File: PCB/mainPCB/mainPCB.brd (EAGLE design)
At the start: 98.7 x 80 mm, 58 parts, among them CN1 SDS-50J, CN2 SDS-50J, CN3 SDS-50J, CN4 SDS-50J, J2 RASPBERRYPI-40-PIN-GPIO, T2 BC817, T3 BC817, T4 BC817, T6 BC817, U1 AT24C256C-SSHL-B, U11 SFH615A-07, U12 ALQ105, U3 SFH615A-07, U4 ALQ105, U5 SFH615A-07, U6 ALQ105, U7 SFH615A-07, U8 ALQ105

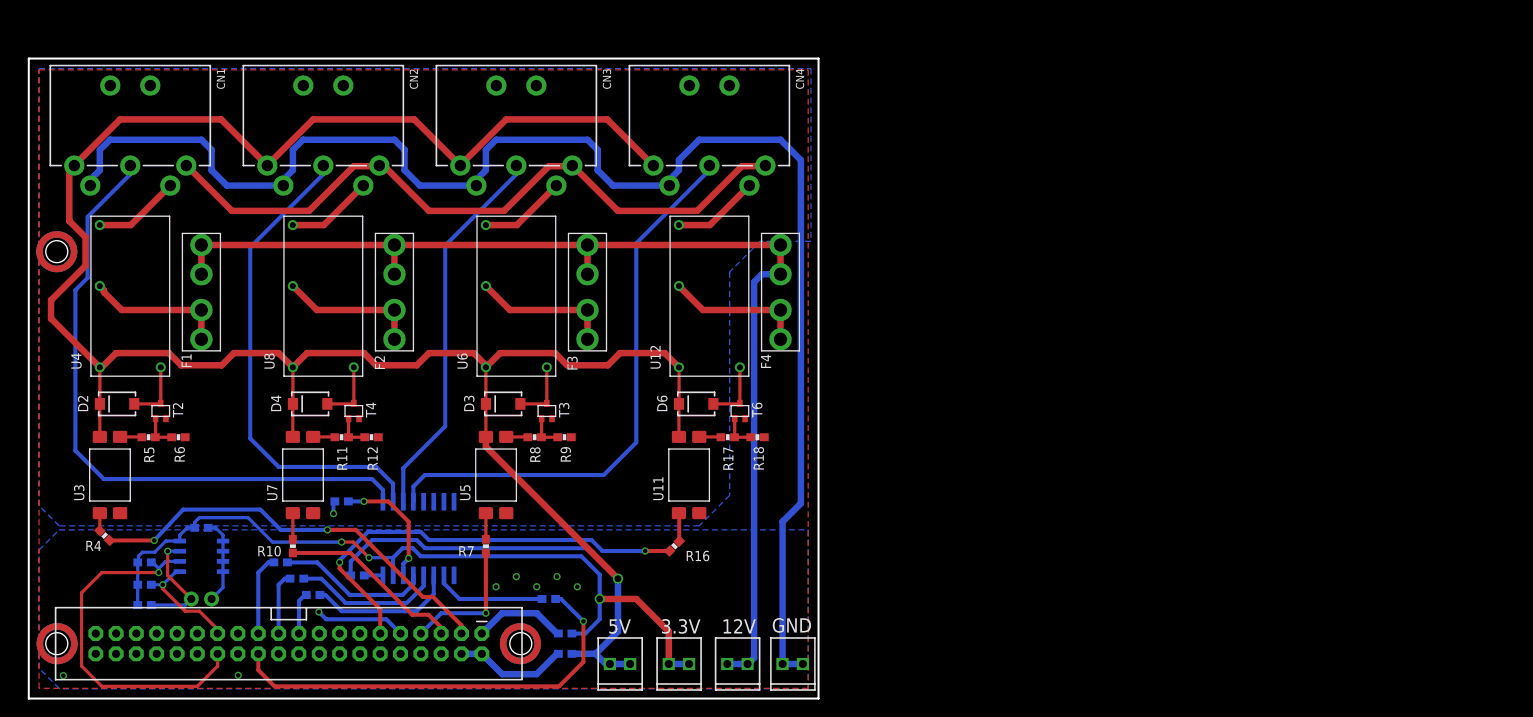
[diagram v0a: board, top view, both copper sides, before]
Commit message: Adding files for v0.2
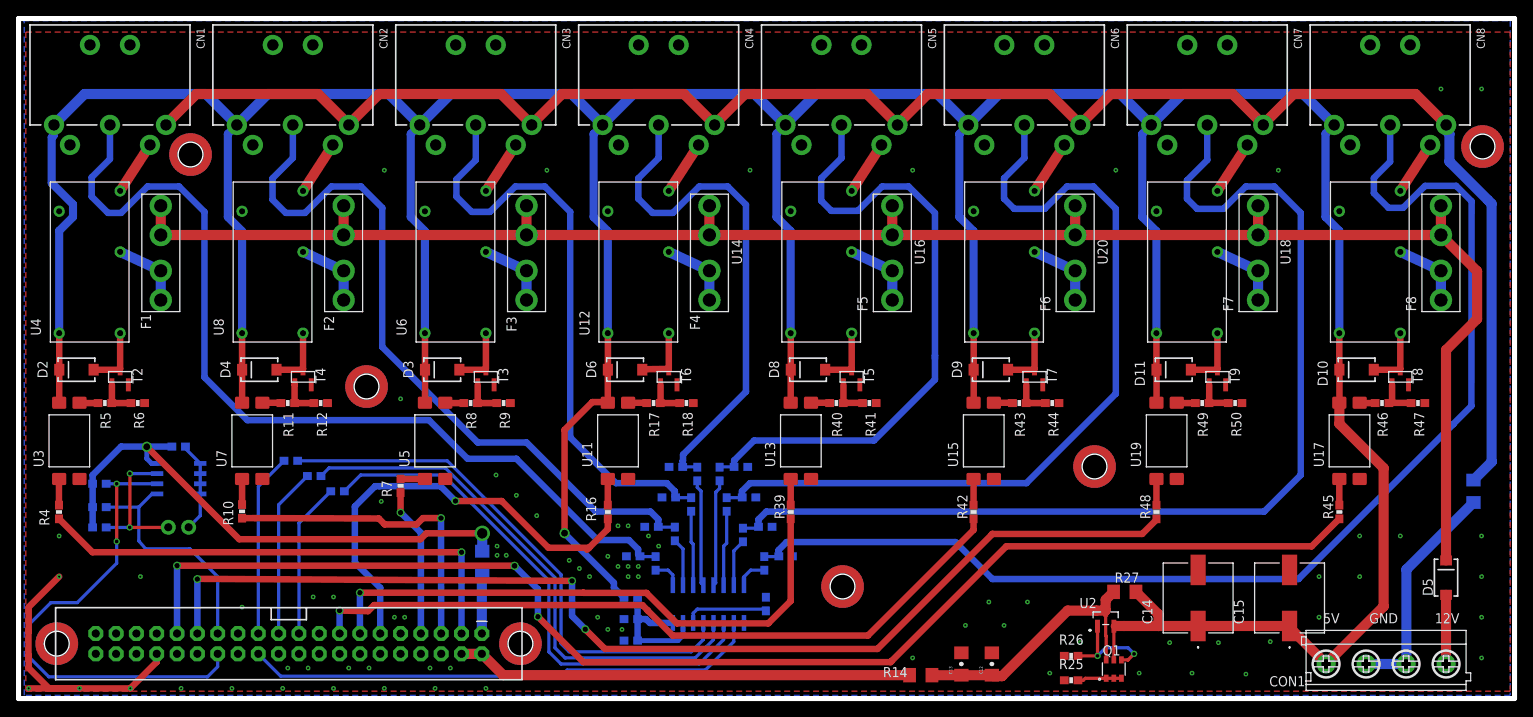
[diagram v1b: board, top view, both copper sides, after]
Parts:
- removed J1, J3, J4, J5: (no value), SparkFun-Connectors:1X02_2.54_SCREWTERM
- removed U$1: MCP3208I/SL, adcLib:SO-16DW
- added C10, C11, C2, C3, C4, C5, C6, C7, C8, C9: 0.1uF, SparkFun-Capacitors:0603-CAP
- added C12, C13: 10uF, SparkFun-Capacitors:1206-CAP
- added C14, C15: EEE-HA1C471UPCAP_PAN_EEE_F-L, EEE-HA1C471UP:CAP_PAN_EEE_F-L
- added CN5, CN6, CN7, CN8: SDS-50J, SDS-50J:SDS-50J
- added CON1: 1776244-4, lib:1776244-4
- added D10, D11, D5, D8, D9: (no value), SparkFun-DiscreteSemi:SMA-DIODE
- added F5, F6, F7, F8: 3544-2, lib:3544-2
- added FRAME3: FRAME-LETTER, SparkFun-Aesthetics:CREATIVE_COMMONS
- added Q1: DMMT5401-7-F, DMMT5401-7-F:SOT26
- added R24: 0, SparkFun-Passives:1206
- added R25, R40, R43, R46, R49: 10k, SparkFun-Passives:0603-RES
- added R26, R41, R44, R47, R50: 47k, SparkFun-Passives:0603-RES
- added R27: DNP, SparkFun-Passives:1206
- added R28, R29, R30, R31, R32, R33, R34, R35: 330, SparkFun-Passives:0603-RES
- added R39, R42, R45, R48: 47, SparkFun-Passives:0603-RES
- added T5, T7, T8, T9: BC817, lib:BC817
- added U$2: MCP3208T-CI/SL, MCP3208T-CI_SL:SOIC16-N_MC
- added U13, U15, U17, U19: SFH615A-07, lib:SFH615A-07
- added U14, U16, U18, U20: ALQ105, lib:ALQ105
- added U2: DMG2305UX-13SOT-23-M, DMG2359UX:SOT-23-M
- R14, R15: device SparkFun-Passives:0603-RES -> SparkFun-Passives:1206
- R21: value 1k -> 3.9k
- moved FRAME2 73.1 mm to (171.1, 3.12)
- moved FRAME1 67.6 mm to (165.7, 3.12)
- moved R20 54.6 mm to (93.4, 11.8), turned to 270 degrees
- moved R14 44.5 mm to (112.8, 2.92), flipped to the top, turned to 180 degrees
- moved R19 34.3 mm to (76.5, 12.6)
- moved U12 18.3 mm to (77.5, 54.6)
- moved U6 17.4 mm to (54.6, 54.6)
- moved U8 16.6 mm to (31.8, 54.6)
- moved U4 15.9 mm to (8.89, 54.6)
- moved R15 13.7 mm to (58.0, 17.0), turned to 270 degrees
- moved R2 13.3 mm to (39.9, 25.9)
- moved R7 13.1 mm to (47.8, 26.6)
- moved R1 13.0 mm to (37.0, 27.8)
- moved R13 12.8 mm to (34.0, 29.7)
- moved R23 11.3 mm to (10.1, 26.8)
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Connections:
- new net 5V_RPI: C12.1, C13.1, Q1.6, R14.1, R27.1, U2.3
- new net A1_F: C2.1, CN1.2, R28.2
- new net A2_F: C3.1, CN2.2, R29.2
- new net A3_F: C4.1, CN3.2, R30.2
- new net A4_F: C5.1, CN4.2, R31.2
- new net A5_F: C6.1, CN5.2, R32.2
- new net A6_F: C7.1, CN6.2, R33.2
- new net A7_F: C8.1, CN7.2, R34.2
- new net A8_F: C9.1, CN8.2, R35.2
- new net N$29: Q1.4, R26.2, U2.1
- new net N$30: CON1.4, D5.A
- new net N$31: F5.P$1, F5.P$2, U14.P$3
- new net N$32: F6.P$1, F6.P$2, U16.P$3
- new net N$33: F7.P$1, F7.P$2, U20.P$3
- new net N$34: F8.P$1, F8.P$2, U18.P$3
- new net N$35: R39.2, U13.P$1
- new net N$36: C10.1, C11.1, R19.1, U$2.15, U$2.16
- new net N$37: R40.2, U13.P$3
- new net N$38: R40.1, R41.2, T5.P$2
- new net N$39: D8.A, T5.P$1, U14.P$2
- new net N$40: R42.2, U15.P$1
- new net N$41: R43.2, U15.P$3
- new net N$42: R43.1, R44.2, T7.P$2
- new net N$43: D9.A, T7.P$1, U16.P$2
- new net N$44: R45.2, U17.P$1
- new net N$45: R46.2, U17.P$3
- new net N$46: R46.1, R47.2, T8.P$2
- new net N$47: D10.A, T8.P$1, U18.P$2
- new net N$48: R48.2, U19.P$1
- new net N$49: R49.2, U19.P$3
- new net N$50: R49.1, R50.2, T9.P$2
- new net N$51: D11.A, T9.P$1, U20.P$2
- new net R5: CN5.5, U14.P$4
- new net R6: CN6.5, U16.P$4
- new net R7: CN7.5, U20.P$4
- new net R8: CN8.5, U18.P$4
- new net RELAY5: J2.13, R39.1
- new net RELAY6: J2.15, R42.1
- new net RELAY7: J2.29, R48.1
- new net RELAY8: J2.31, R45.1
- net 12V: now also D5.C, F5.P$3, F5.P$4, F6.P$3, F6.P$4, F7.P$3, F7.P$4, F8.P$3, F8.P$4; no longer J4.P1, J4.P2
- net 3_3V: no longer J1.P1, J1.P2, U$1.15
- net 5V: now also C14.1, C15.1, CN5.1, CN6.1, CN7.1, CN8.1, CON1.1, D10.C, D11.C, D8.C, D9.C, Q1.5, R27.2, U12.P$1, U13.P$4, U14.P$1, U15.P$4, U16.P$1, U17.P$4, U18.P$1, U19.P$4, U2.2, U20.P$1, U4.P$1, U6.P$1, U8.P$1; no longer J3.P1, J3.P2, R14.1, U12.P$2, U4.P$2, U6.P$2, U8.P$2
- net A1: now also R28.1, U$2.1; no longer CN1.2, U$1.1
- net A2: now also R29.1, U$2.2; no longer CN2.2, U$1.2
- net A3: now also R30.1, U$2.3; no longer CN3.2, U$1.3
- net A4: now also R31.1, U$2.4; no longer CN4.2, U$1.4
- net A5: now also R32.1, U$2.5; no longer U$1.5
- net A6: now also R33.1, U$2.6; no longer U$1.6
- net A7: now also R34.1, U$2.7; no longer U$1.7
- net A8: now also R35.1, U$2.8; no longer U$1.8
- net AGND: now also U$2.14; no longer U$1.14
- net CLK: now also U$2.13; no longer U$1.13
- net COM: now also CN5.3, CN6.3, CN7.3, CN8.3, R24.1
- net CS_ADC: now also U$2.10; no longer U$1.10
- net GND: now also C10.2, C11.2, C12.2, C13.2, C14.2, C15.2, C2.2, C3.2, C4.2, C5.2, C6.2, C7.2, C8.2, C9.2, CN5.4, CN6.4, CN7.4, CN8.4, CON1.2, CON1.3, R24.2, R25.1, R26.1, R41.1, R44.1, R47.1, R50.1, T5.P$3, T7.P$3, T8.P$3, T9.P$3, U$2.9, U13.P$2, U15.P$2, U17.P$2, U19.P$2; no longer J5.P1, J5.P2, U$1.9
- net MISO: now also U$2.12; no longer U$1.12
- net MOSI: now also U$2.11; no longer U$1.11
- net N$12: now also U6.P$2; no longer U6.P$1
- net N$16: now also U8.P$2; no longer U8.P$1
- net N$24: now also U12.P$2; no longer U12.P$1
- net N$27: now also Q1.1, Q1.2, Q1.3, R25.2; no longer R19.1, U$1.16
- net N$8: now also U4.P$2; no longer U4.P$1
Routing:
- net 5V: track 314.2 -> 578.8 mm
- net RELAY8: track 0.00 -> 168.2 mm, vias 0 -> 3
- net A8_F: track 0.00 -> 150.4 mm
- net COM: track 86.5 -> 230.3 mm
- net RELAY7: track 0.00 -> 139.7 mm, vias 0 -> 3
- net A7_F: track 0.00 -> 133.3 mm
- net GND: track 208.1 -> 78.9 mm, vias 9 -> 78
- net A1_F: track 0.00 -> 114.3 mm
- net A6_F: track 0.00 -> 104.7 mm
- net 12V: track 141.7 -> 233.5 mm
- net A2_F: track 0.00 -> 91.1 mm
- net RELAY6: track 0.00 -> 90.9 mm, vias 0 -> 1
- net A5_F: track 0.00 -> 81.2 mm
- net A1: track 80.4 -> 3.69 mm
- net A3_F: track 0.00 -> 74.4 mm
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- removed copper zone on layer 16, net AGND
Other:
- board size 98.7 x 80 mm -> 187 x 85 mm
- board text added: "v0.2"
- board text removed: "3.3V"
- board text removed: "v0.1"
